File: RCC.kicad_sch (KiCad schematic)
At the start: 44 parts, among them J1 Battery, J2 USB_C_Receptacle_USB2.0_16P, J3 Conn_01x07, J4 Conn_01x04_Pin, SW2 SW_Push, U1 BQ24040DGQR, U2 ESD7104MUTAG, U3 TLV75801PDRV, U5 STM32L412KBTx, Y1 ECS-2520MVQ-480-CN-TR

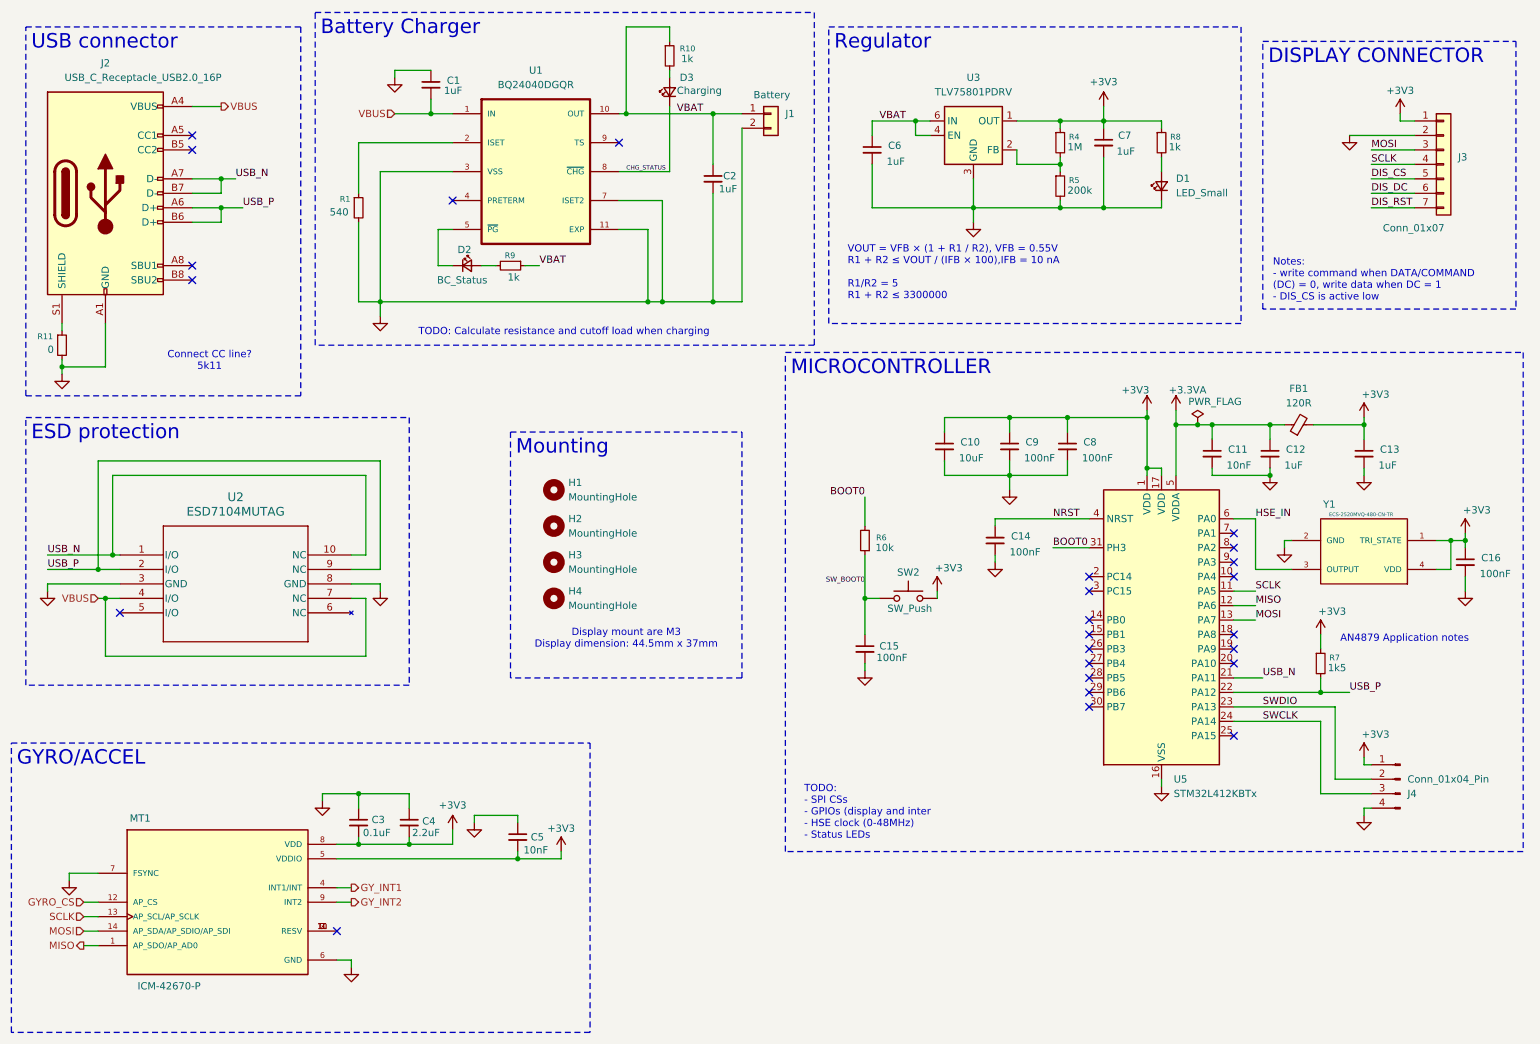
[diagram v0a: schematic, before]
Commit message: Finalise PCB and add 3d models
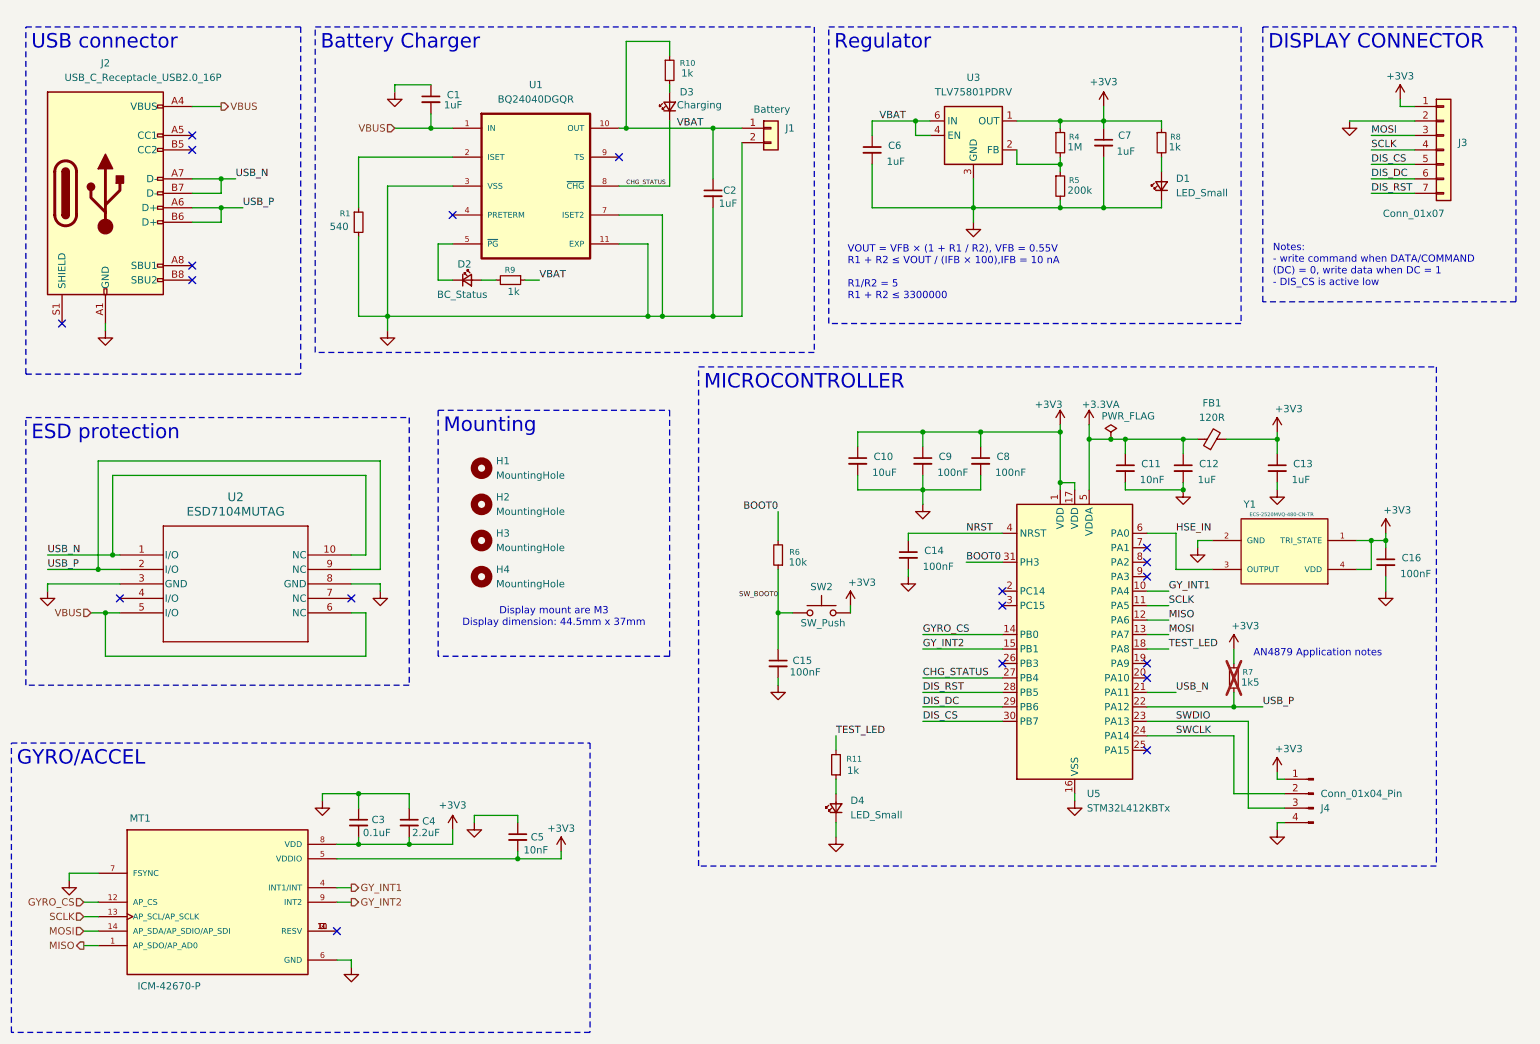
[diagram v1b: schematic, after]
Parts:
- added D4: LED_Small, LED_SMD:LED_0603_1608Metric, symbol Device:LED_Small
- J4: footprint Connector_JST:JST_EH_B4B-EH-A_1x04_P2.50mm_Vertical -> Connector_JST:JST_EH_S4B-EH_1x04_P2.50mm_Horizontal
- R11: value 0 -> 1k
- R7: now not fitted
- U2: footprint ESD7104:UDFN10_ONS -> UDFN10_ONS
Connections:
- net CHG_STATUS: now also U5.27 (PB4)
- net DIS_CS: now also U5.30 (PB7)
- net DIS_DC: now also U5.29 (PB6)
- net DIS_RST: now also U5.28 (PB5)
- net GND: now also D4.1 (K); no longer R11.2
- net GYRO_CS: now also U5.14 (PB0)
- net GY_INT1: now also U5.10 (PA4)
- net GY_INT2: now also U5.15 (PB1)
- net SWCLK: now also J4.2 (Pin_2); no longer J4.3 (Pin_3)
- net SWDIO: now also J4.3 (Pin_3); no longer J4.2 (Pin_2)
- net VBUS: now also U2.5 (I/O), U2.6 (NC); no longer U2.4 (I/O), U2.7 (NC)
- net at J2.S1 (SHIELD): no longer R11.1
- net TEST_LED: now reaches U5.18 (PA8)
- net TEST_LED: now also R11.2
- new net: D4.2 (A), R11.1
- no-connect marks 25 -> 19
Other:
- note removed: "Connect CC line? 5k11"
- note removed: "TODO: - SPI CSs - GPIOs (display and inter - HSE clock (0-48MHz) - Status LEDs"
- note removed: "TODO: Calculate resistance and cutoff load when charging"
- moved on the sheet: C1, C10, C11, C12, C13, C14, C15, C16, C2, C8, C9, D2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
